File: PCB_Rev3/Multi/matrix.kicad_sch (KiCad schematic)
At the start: 159 parts

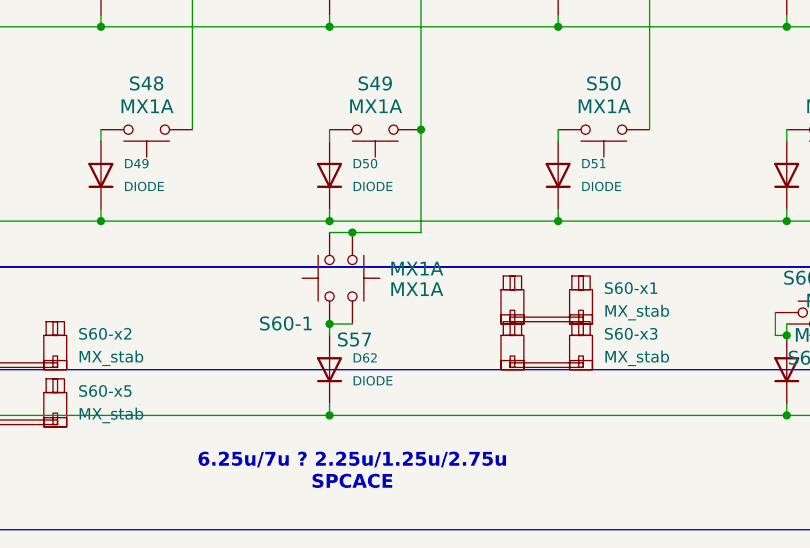
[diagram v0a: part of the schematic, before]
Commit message: 6u空格添加，卫星轴修改
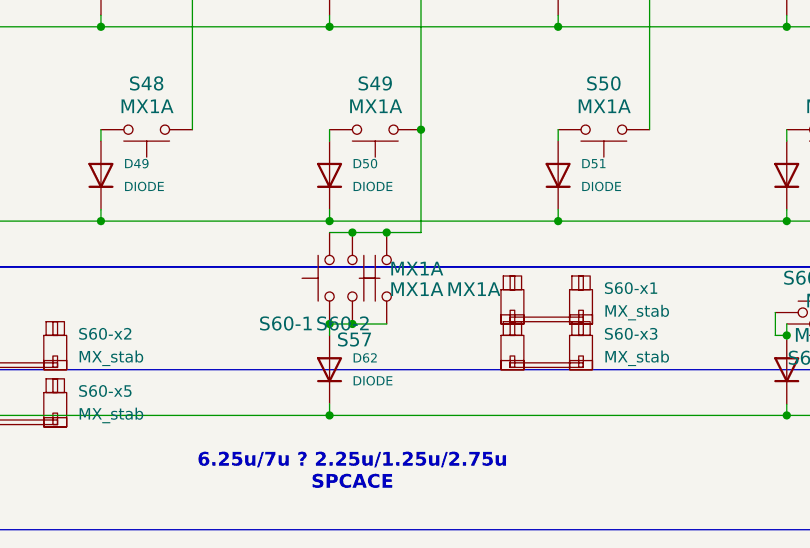
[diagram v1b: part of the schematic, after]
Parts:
- added S60-2: MX1A, PCM_Switch_Keyboard_Hotswap_Kailh:SW_Hotswap_Kailh_MX_Plated_6.25u, symbol Switch:SW_Push
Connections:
- net col_6: now also S60-2.1
- net at D62.2 (A), S57.1, S60-1.2: now also S60-2.2
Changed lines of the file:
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@@
 	)
 	(junction
+		(at 198.12 147.32)
+		(diameter 0)
+		(color 0 0 0 0)
+	)
+	(junction
 		(at 53.34 102.87)
 		(diameter 0)
@@
 	)
 	(junction
+		(at 201.93 137.16)
+		(diameter 0)
+		(color 0 0 0 0)
+	)
+	(junction
 		(at 358.14 82.55)
 		(diameter 0)
@@
 	(wire
 		(pts
+			(xy 201.93 137.16) (xy 205.74 137.16)
+		)
+		(stroke
+			(width 0)
+			(type default)
+		)
+	)
+	(wire
+		(pts
 			(xy 170.18 113.03) (xy 170.18 114.3)
 		)
@@
 	(wire
 		(pts
-			(xy 198.12 137.16) (xy 205.74 137.16)
+			(xy 198.12 137.16) (xy 201.93 137.16)
 		)
 		(stroke
@@
 	(wire
 		(pts
+			(xy 198.12 147.32) (xy 201.93 147.32)
+		)
+		(stroke
+			(width 0)
+			(type default)
+		)
+	)
+	(wire
+		(pts
 			(xy 195.58 135.89) (xy 220.98 135.89)
 		)
@@
 					(unit 1)
 				)
+			)
+		)
+	)
+	(symbol
+		(lib_id "Switch:SW_Push")
+		(at 201.93 142.24 90)
+		(mirror x)
+		(unit 1)
+		(exclude_from_sim no)
+		(in_bom yes)
+		(on_board yes)
+		(dnp no)
+		(property "Reference" "S60-2"
+			(at 197.104 147.32 90)
+			(effects
+				(font
+					(size 1.524 1.524)
+				)
+			)
+		)
+		(property "Value" "MX1A"
+			(at 211.582 143.51 90)
+			(effects
+				(font
+					(size 1.524 1.524)
+				)
+			)
+		)
+		(property "Footprint" "PCM_Switch_Keyboard_Hotswap_Kailh:SW_Hotswap_Kailh_MX_Plated_6.25u"
+			(at 196.85 142.24 0)
+			(effects
+				(font
+					(size 1.27 1.27)
+				)
+				(hide yes)
+			)
+		)
+		(property "Datasheet" "~"
+			(at 196.85 142.24 0)
+			(effects
+				(font
+					(size 1.27 1.27)
+				)
+				(hide yes)
+			)
+		)
+		(property "Description" "Push button switch, generic, two pins"
+			(at 201.93 142.24 0)
+			(effects
+				(font
+					(size 1.27 1.27)
+				)
+				(hide yes)
+			)
+		)
+		(pin "2"
+		)
+		(pin "1"
+		)
+		(instances
+			(project "PH60_Rev3"
+				(path "/dca0f898-8fdb-4522-a51d-f4f4238906e7/dc5cd3b2-ef82-41de-b720-71645d542746"
+					(reference "S60-2")
+					(unit 1)
+				)
